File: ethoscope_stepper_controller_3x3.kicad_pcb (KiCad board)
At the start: 2 copper layers, 74.9 x 74.9 mm, 69 parts, among them P1 PWR_JACK_2.1x5.5_SMD_VERT, T1 TERM_BLK, T2 TERM_BLK, T3 TERM_BLK, T4 TERM_BLK, T5 TERM_BLK, T6 TERM_BLK, T7 TERM_BLK, U1 TMC429, U10 DRV8846, U11 TMC429, U12 BUFFER_TRI_STATE, U13 DRV8846, U2 BUFFER_TRI_STATE, U3 DRV8846, U4 DRV8846, U5 DRV8846, U6 TMC429, U7 BUFFER_TRI_STATE, U8 DRV8846, U9 DRV8846

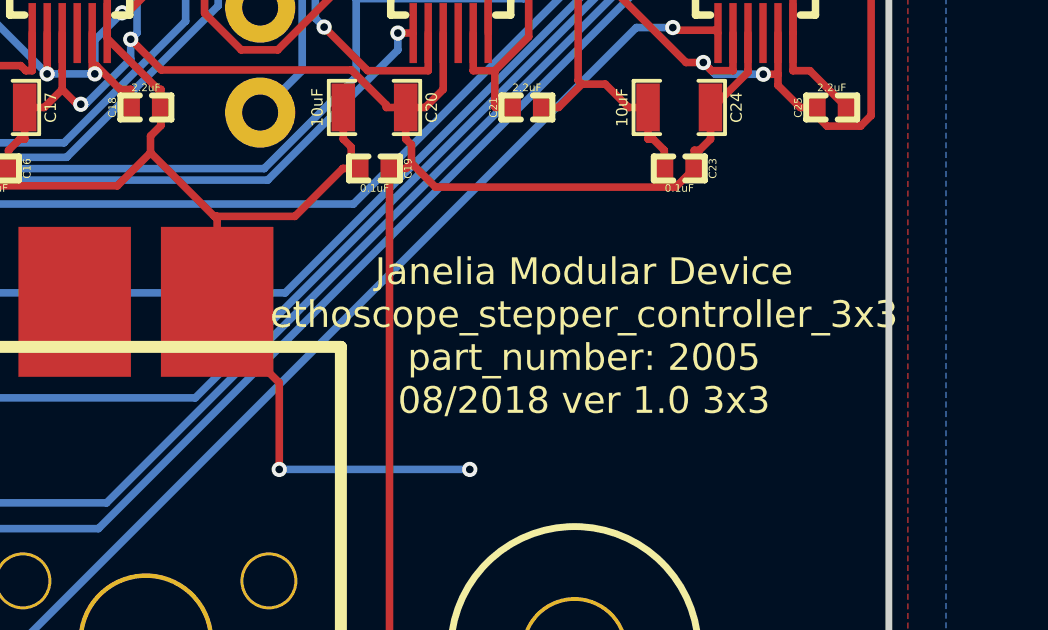
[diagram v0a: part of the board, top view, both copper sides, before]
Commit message: Finished version 1.0.
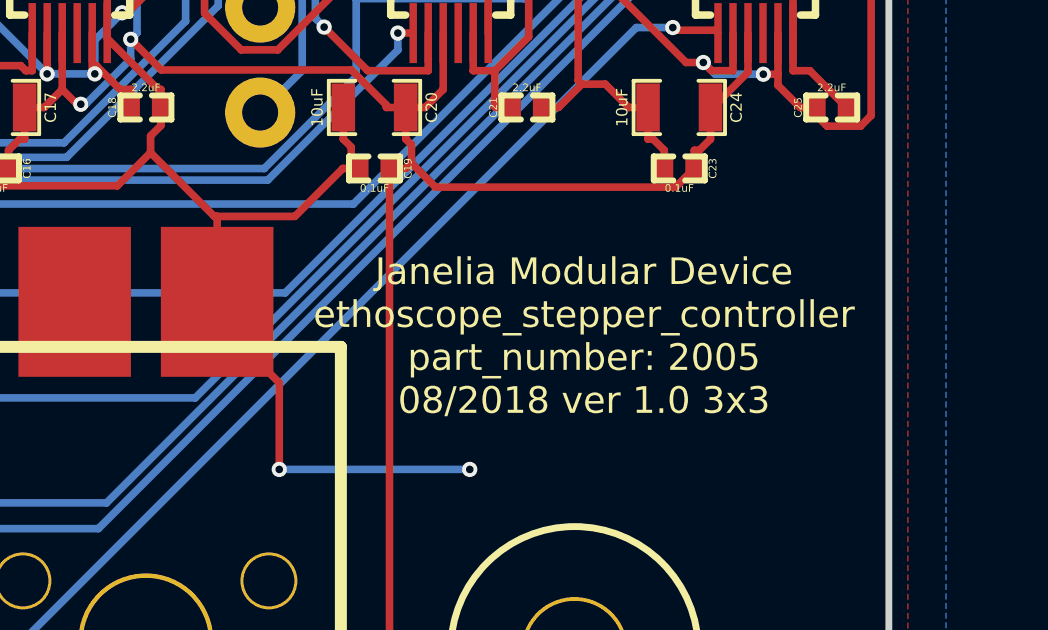
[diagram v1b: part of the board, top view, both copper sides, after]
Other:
- board text added: "Janelia Modular Device ethoscope_stepper_controller part_number: 2005 08/2018 ver 1.0 3x3"
- board text removed: "Janelia Modular Device ethoscope_stepper_controller_3x3 part_number: 2005 08/2018 ver 1.0 3x3"
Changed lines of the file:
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@@
     (effects (font (size 1.016 1.016) (thickness 0.1905)))
   )
-  (gr_text "Janelia Modular Device\nethoscope_stepper_controller_3x3\npart_number: 2005\n08/2018 ver 1.0 3x3" (at 179.705 118.11) (layer F.SilkS)
+  (gr_text "Janelia Modular Device\nethoscope_stepper_controller\npart_number: 2005\n08/2018 ver 1.0 3x3" (at 179.705 118.11) (layer F.SilkS)
     (effects (font (size 0.889 0.889) (thickness 0.22225)))
   )

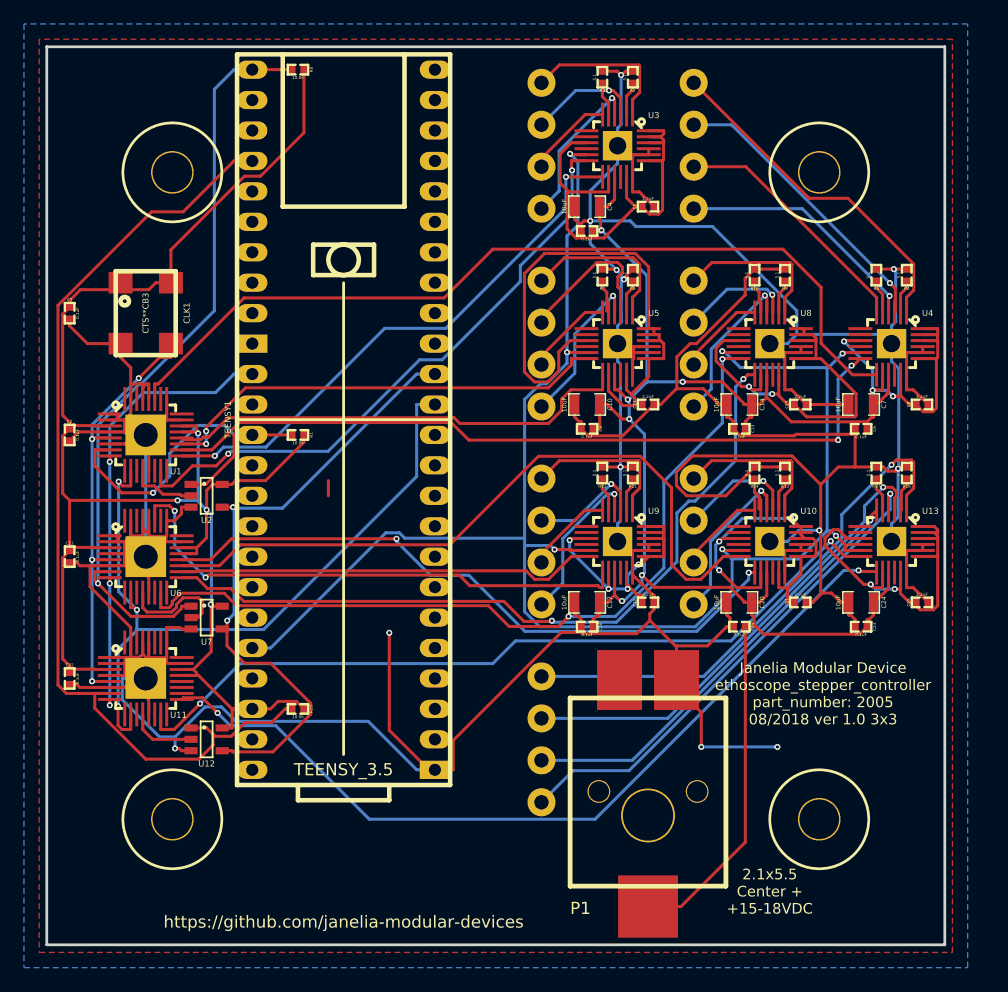
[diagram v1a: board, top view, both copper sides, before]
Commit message: Rearranged schematics.
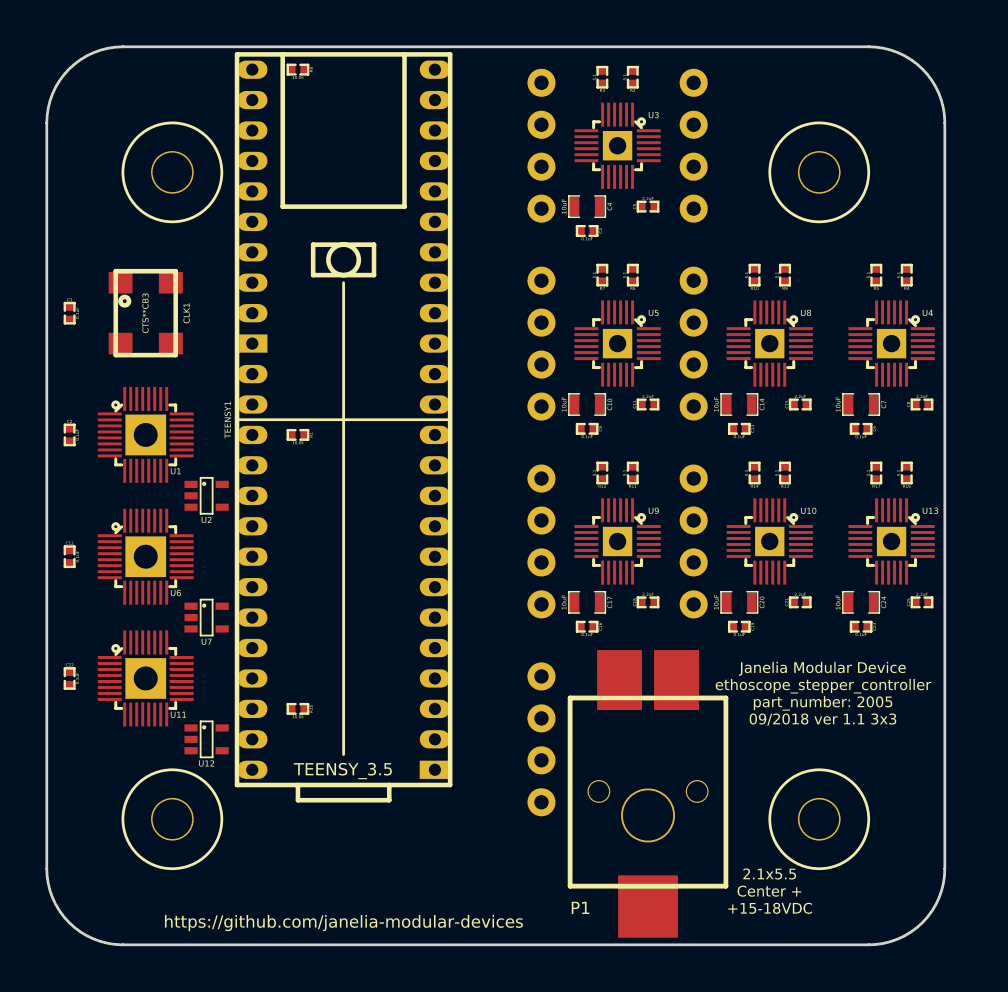
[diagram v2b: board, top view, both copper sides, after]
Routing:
- net GND: track 490.5 -> 0.00 mm, vias 12 -> 0
- net VAA: track 145.8 -> 0.00 mm, vias 6 -> 0
- net +3V3: track 145.4 -> 0.00 mm, vias 4 -> 0
- net /ENABLE_ALL: track 140.4 -> 0.00 mm, vias 7 -> 0
- net /CS_429_2: track 81.4 -> 0.00 mm
- net /tmc429_0/DIR_1: track 73.2 -> 0.00 mm
- net /tmc429_2/DIR_0: track 70.9 -> 0.00 mm, vias 2 -> 0
- net /tmc429_1/STEP_0: track 67.9 -> 0.00 mm, vias 2 -> 0
- net /tmc429_2/STEP_0: track 66.7 -> 0.00 mm, vias 2 -> 0
- net /MOSI: track 64.5 -> 0.00 mm, vias 3 -> 0
- net /CS_429_1: track 64.2 -> 0.00 mm, vias 1 -> 0
- net /tmc429_0/STEP_1: track 64.0 -> 0.00 mm, vias 2 -> 0
- net /tmc429_1/DIR_0: track 63.9 -> 0.00 mm, vias 2 -> 0
- net /tmc429_1/STEP_2: track 59.1 -> 0.00 mm
- net /tmc429_1/DIR_2: track 54.2 -> 0.00 mm, vias 2 -> 0
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- removed copper zone on B.Cu, net GND
- removed copper zone on F.Cu, net GND
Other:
- outline, holes or cut-outs redrawn
- board text added: "Janelia Modular Device ethoscope_stepper_controller part_number: 2005 09/2018 ver 1.1 3x3"
- board text removed: "Janelia Modular Device ethoscope_stepper_controller part_number: 2005 08/2018 ver 1.0 3x3"
